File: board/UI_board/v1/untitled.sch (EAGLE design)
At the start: 21 parts, among them X1 JST-XH-02-PIN-ROUND-PAD

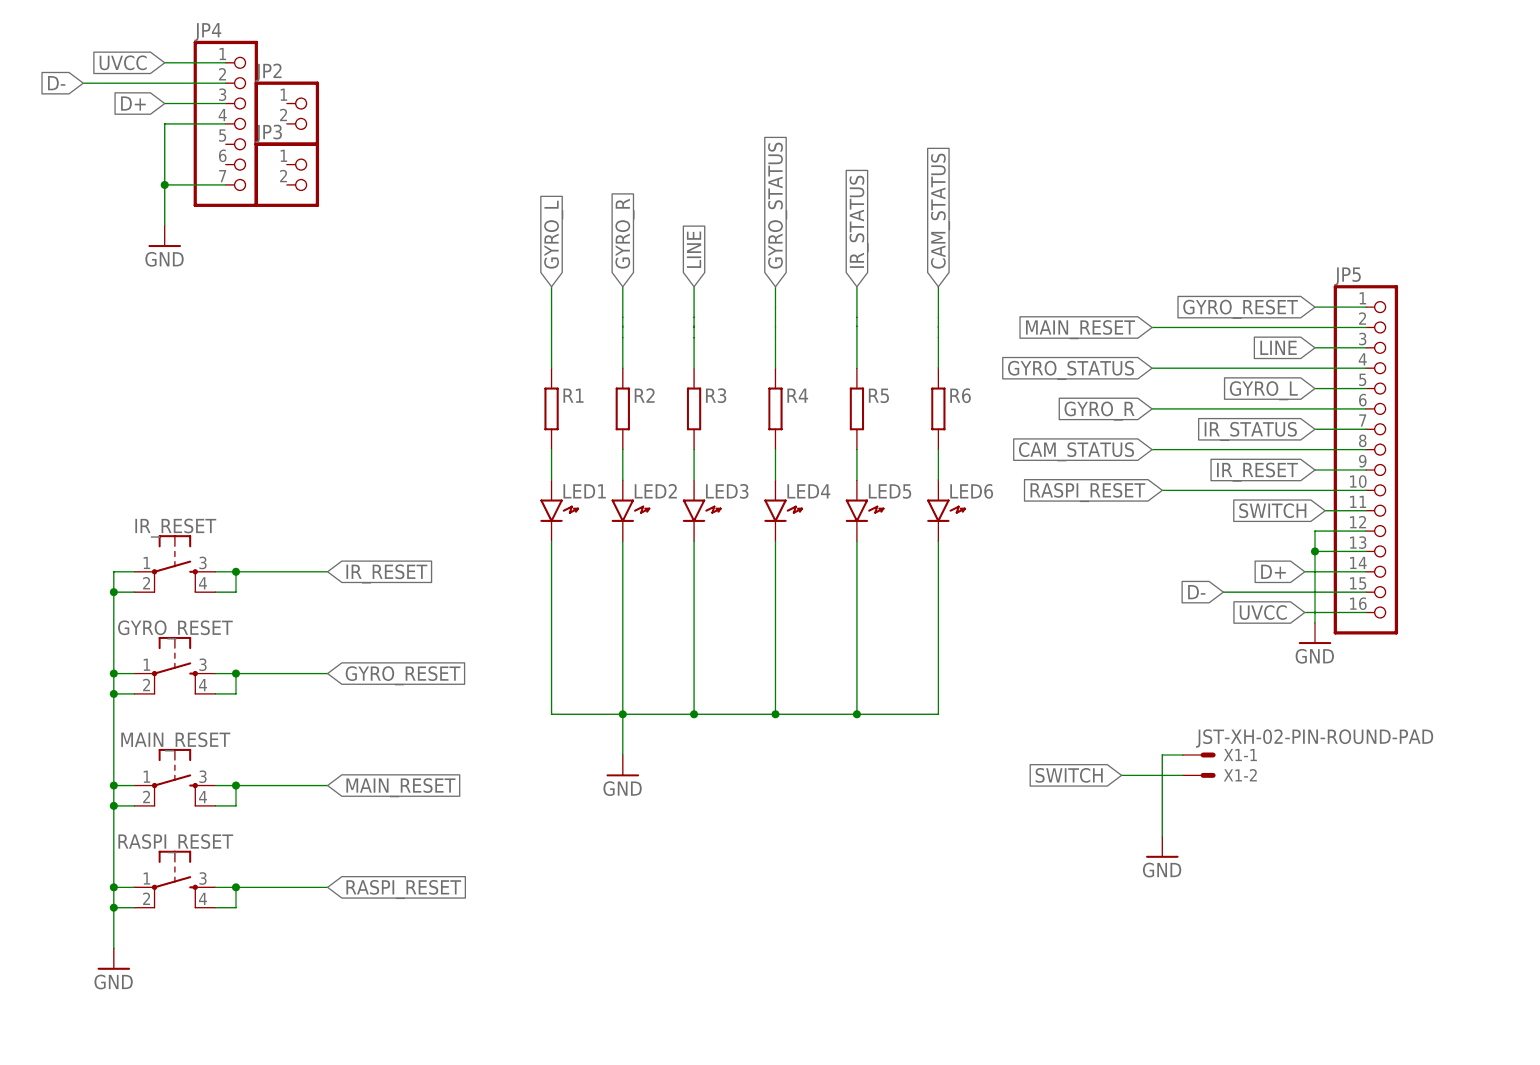
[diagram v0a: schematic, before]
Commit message: marge前のファイル
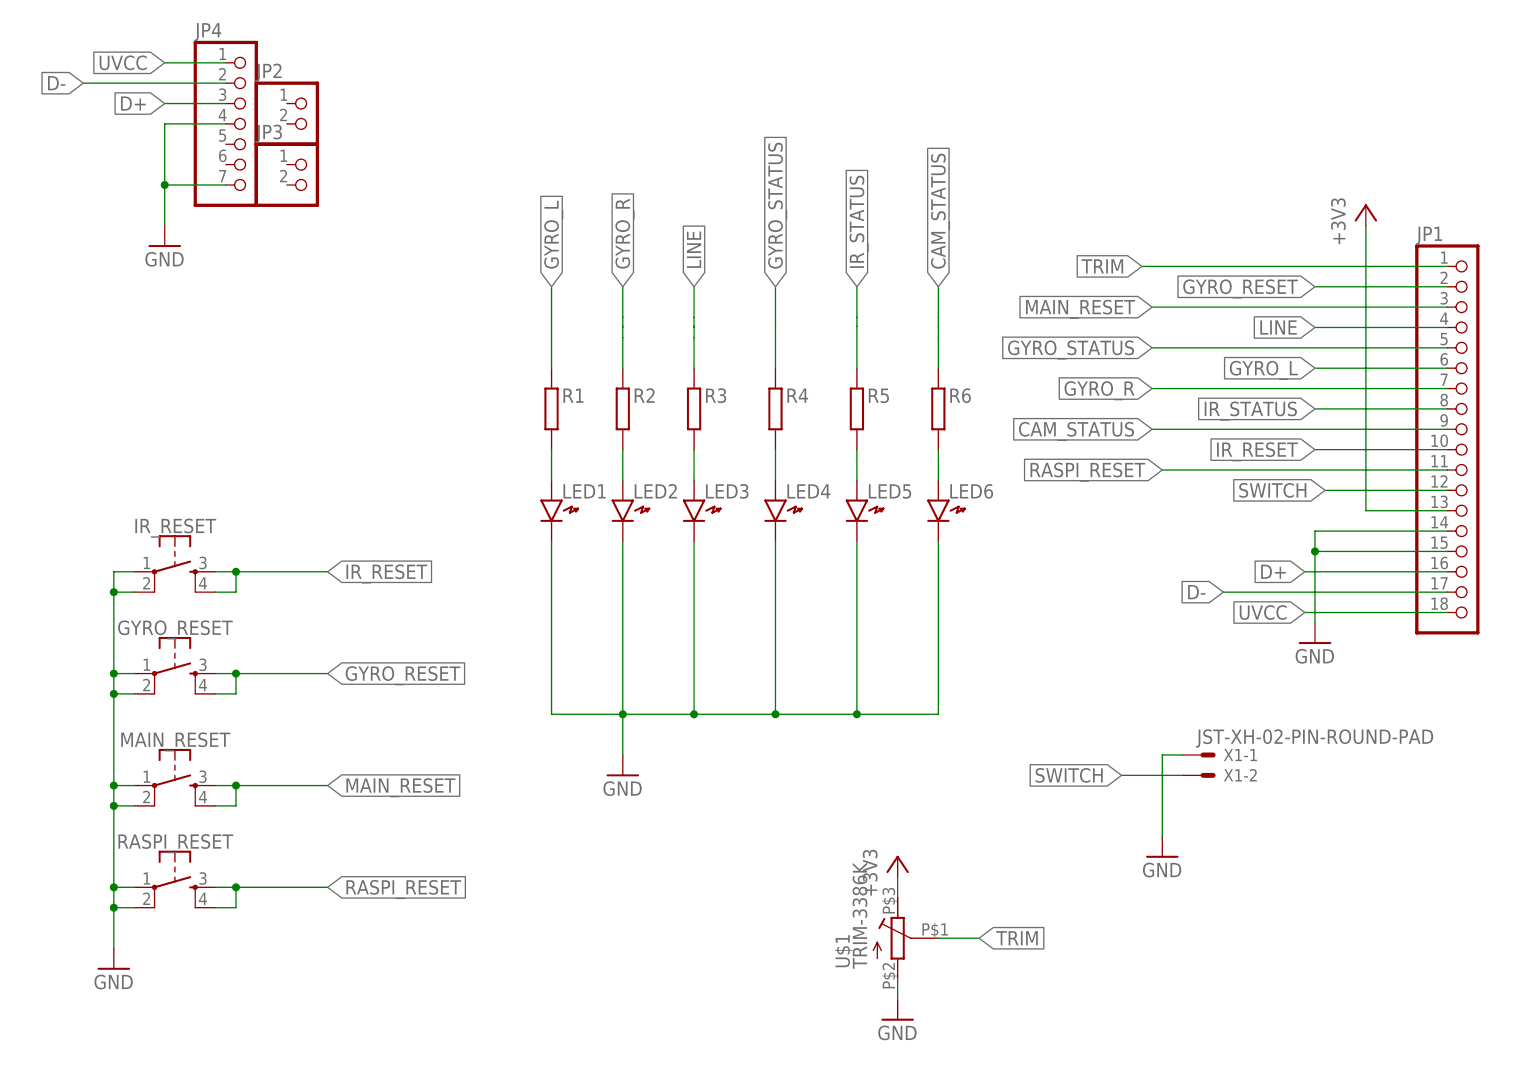
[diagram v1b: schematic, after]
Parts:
- removed JP5: (no value), pinhead:PINHD-1X16
- added JP1: (no value), pinhead:PINHD-1X18
- added U$1: TRIM-3386K, R-trim:TRIM-3386K
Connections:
- new net +3V3: JP1.13, U$1.1
- new net TRIM: JP1.1, U$1.3
- net CAM_STATUS: now also JP1.9; no longer JP5.8
- net D+: now also JP1.16; no longer JP5.14
- net D-: now also JP1.17; no longer JP5.15
- net GND: now also JP1.14, JP1.15, U$1.2; no longer JP5.12, JP5.13
- net GYRO_L: now also JP1.6; no longer JP5.5
- net GYRO_R: now also JP1.7; no longer JP5.6
- net GYRO_RESET: now also JP1.2; no longer JP5.1
- net GYRO_STATUS: now also JP1.5; no longer JP5.4
- net IR_RESET: now also JP1.10; no longer JP5.9
- net IR_STATUS: now also JP1.8; no longer JP5.7
- net LINE: now also JP1.4; no longer JP5.3
- net MAIN_RESET: now also JP1.3; no longer JP5.2
- net RASPI_RESET: now also JP1.11; no longer JP5.10
- net SWITCH: now also JP1.12; no longer JP5.11
- net UVCC: now also JP1.18; no longer JP5.16
